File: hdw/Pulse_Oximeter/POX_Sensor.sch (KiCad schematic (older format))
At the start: 2 parts

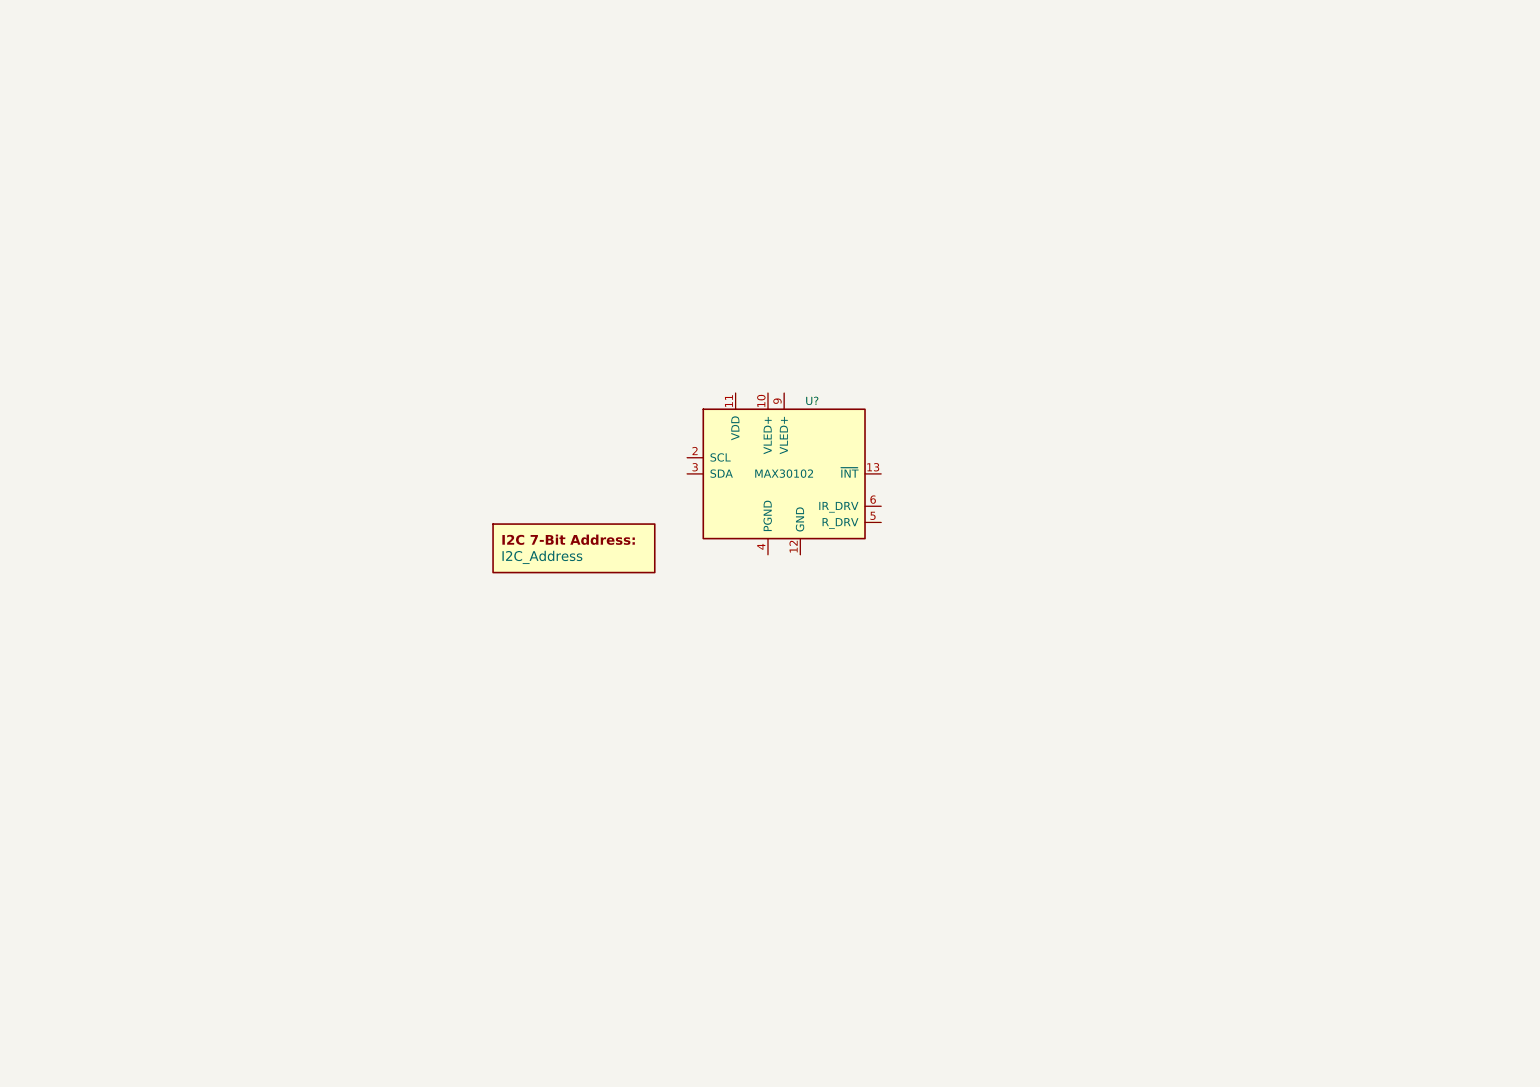
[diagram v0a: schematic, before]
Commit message: Continued schematic development
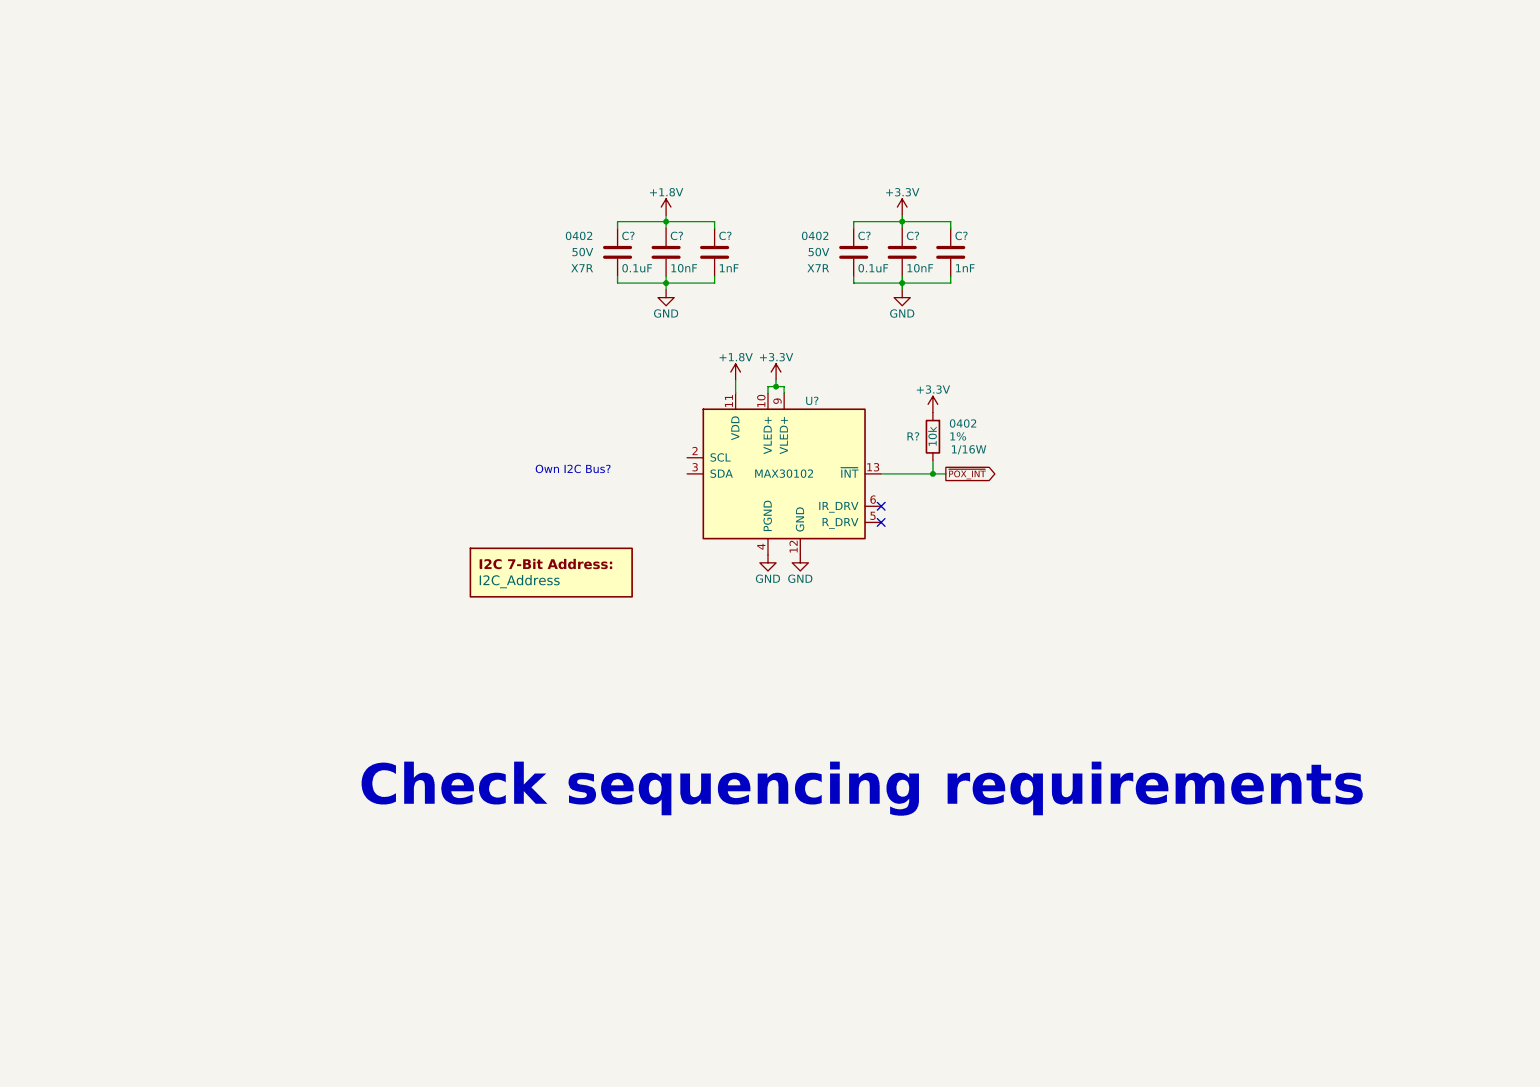
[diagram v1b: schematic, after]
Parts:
- added C? (x2): 0.1uF, Capacitors_SMD:C_0402, symbol Custom_Library:C_Custom
- added C? (x2): 10nF, Capacitors_SMD:C_0402, symbol Custom_Library:C_Custom
- added C? (x2): 1nF, Capacitors_SMD:C_0402, symbol Custom_Library:C_Custom
- added R?: 10k, Resistors_SMD:R_0402, symbol Custom_Library:R_Custom
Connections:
- net +3V3: now reaches U?.10 (VLED+)
- net +3V3: now also U?.9 (VLED+), C?.1, C?.1, C?.1, R?.1
- net +1.8V: now reaches U?.11 (VDD)
- net +1.8V: now also C?.1, C?.1, C?.1
- net GND: now reaches U?.12 (GND)
- net GND: now also U?.4 (PGND), C?.2, C?.2, C?.2, C?.2, C?.2, C?.2
- net ~POX_INT: now reaches U?.13 (~INT)
- net ~POX_INT: now also R?.2
- no-connect marks 0 -> 2
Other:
- note added: "Check sequencing requirements"
- note added: "Own I2C Bus?"

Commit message: few sch additions
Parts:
- added C? (x2): 10uF, Capacitors_SMD:C_0402, symbol Custom_Library:C_Custom
- added U?: TPS22929D, Package_TO_SOT_SMD:SOT-23-6, symbol Power_Management:TPS22929D
- DOC?: value I2C_Address -> 0x57
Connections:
- net labels added: +3.3V_SW
- wire segments 33 -> 36
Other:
- note added: "Own I2C Bus?\nLook at pulup voltage"
- note removed: "Check sequencing requirements"
- note removed: "Own I2C Bus?"
- moved on the sheet: C?, R?, U?

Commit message: More sch work
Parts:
- added C? (x3): 10uF, Capacitors_SMD:C_0402, symbol Custom_Library:C_Custom
- added C? (x2): 0.1uF, Capacitors_SMD:C_0402, symbol Custom_Library:C_Custom
- added R? (x4): 10k, Resistors_SMD:R_0402, symbol Custom_Library:R_Custom
- added U?: TCA9803, Package_SO:VSSOP-8_3.0x3.0mm_P0.65mm, symbol Interface:TCA9803
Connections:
- net labels added: +3.3V_POX, I2C_SCL, I2C_SDA, POS3P3_POX_Enable, POX_I2C_Enable
- net labels removed: +3.3V_SW
- wire segments 36 -> 56
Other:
- note removed: "Own I2C Bus?\nLook at pulup voltage"
- moved on the sheet: C?, R?, U?

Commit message: Added more stuff to sch
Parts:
- R? (x2): Digi-Key PN (none) -> RMCF0402FT10K0CT-ND
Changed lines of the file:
@@
 $Descr A 11000 8500
 encoding utf-8
-Sheet 15 19
-Title ""
+Sheet 15 20
+Title "Pulse Oximeter"
 Date "2020-05-02"
-Rev ""
-Comp ""
+Rev "A"
+Comp "Drew Maatman"
 Comment1 ""
 Comment2 ""
@@
 F 6 "1/16W" H 5850 3630 50  0000 L CNN "Wattage"
 F 7 "DNP" H 5840 3860 50  0000 L CNN "Configuration"
+F 8 "RMCF0402FT10K0CT-ND" H 5740 3710 50  0001 C CNN "Digi-Key PN"
 	1    5740 3710
 	1    0    0    -1
@@
 F 6 "1/16W" H 4980 3630 50  0000 L CNN "Wattage"
 F 7 "DNP" H 4970 3860 50  0000 L CNN "Configuration"
+F 8 "RMCF0402FT10K0CT-ND" H 4870 3710 50  0001 C CNN "Digi-Key PN"
 	1    4870 3710
 	1    0    0    -1

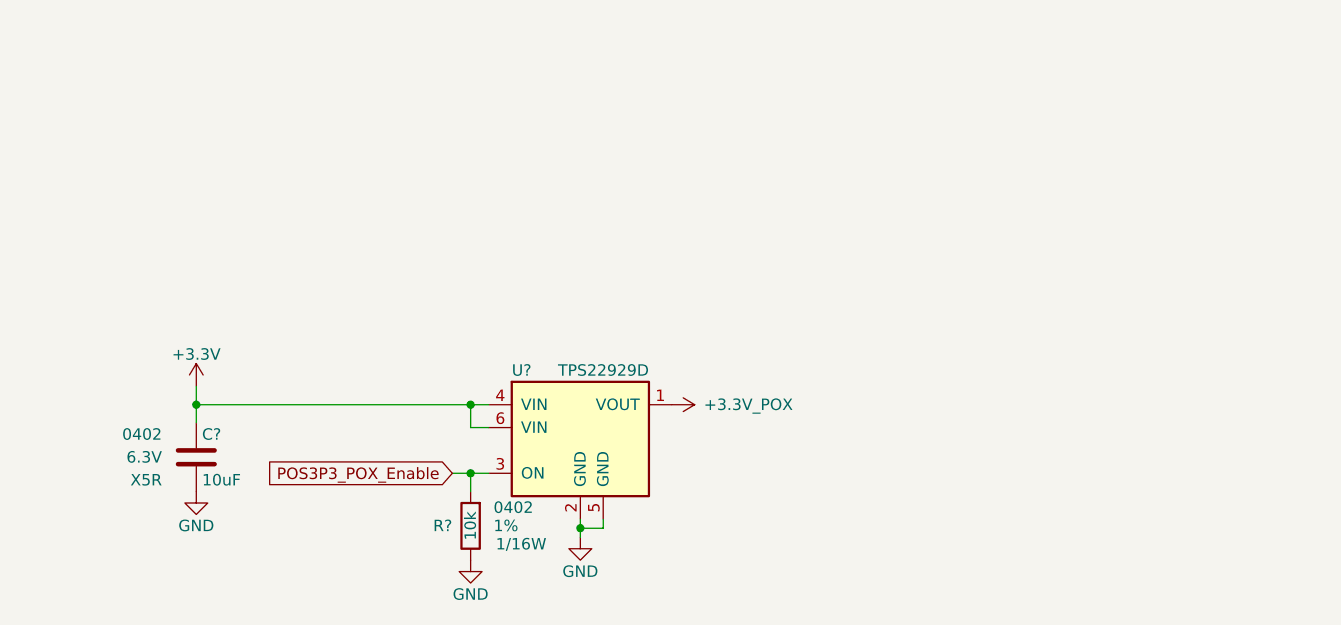
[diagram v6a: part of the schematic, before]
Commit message: Added mech sheet, more complicated bullshit you dont need
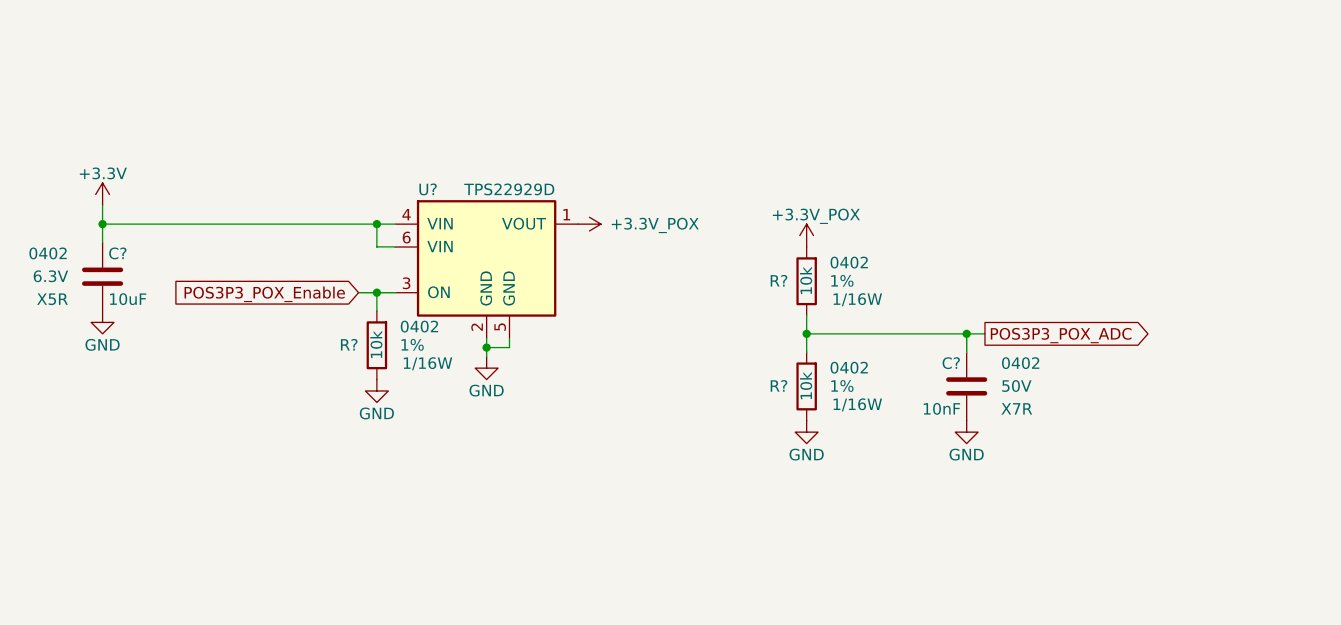
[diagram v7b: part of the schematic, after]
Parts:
- added C?: 10nF, Capacitors_SMD:C_0402, symbol Custom_Library:C_Custom
- added R? (x2): 10k, Resistors_SMD:R_0402, symbol Custom_Library:R_Custom
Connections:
- net +3.3V_POX: now also R?.1
- net GND: now also C?.2, R?.2
- new net POS3P3_POX_ADC: C?.1, R?.1, R?.2
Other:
- moved on the sheet: C?, R?, U?
